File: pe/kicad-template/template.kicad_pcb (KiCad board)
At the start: 2 copper layers, 3 parts

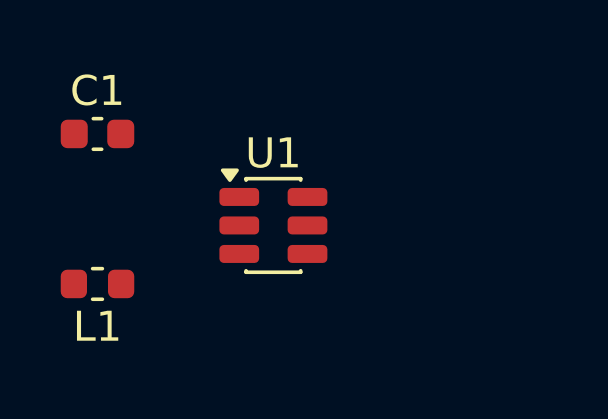
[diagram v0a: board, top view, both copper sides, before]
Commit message: Updated schematic
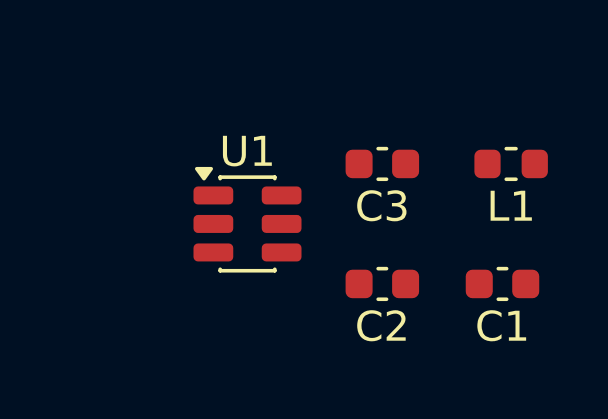
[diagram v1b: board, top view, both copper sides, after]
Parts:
- added C2: 1uF, Capacitor_SMD:C_0603_1608Metric, F.Cu at (146.0, 99.5)
- added C3: 10uF, Capacitor_SMD:C_0603_1608Metric, F.Cu at (146.0, 95.5)
- U1: value ~ -> TPS542025DDCR
- moved C1 14.4 mm to (150.0, 99.5), turned to 180 degrees
- moved L1 14.4 mm to (150.3, 95.5)
- moved U1 0.86 mm to (141.5, 97.5)
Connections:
- C1 pad 2: +5V -> GND
- U1 pad 1: +5V -> GND
- U1 pad 4: unconnected-(U1-FB-Pad4) -> +5V
- U1 pad 6: unconnected-(U1-VBST-Pad6) -> Net-(U1-VBST)
